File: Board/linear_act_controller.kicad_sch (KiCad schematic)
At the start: 16 parts, among them J3 PROG, U1 STM32F030K6Tx

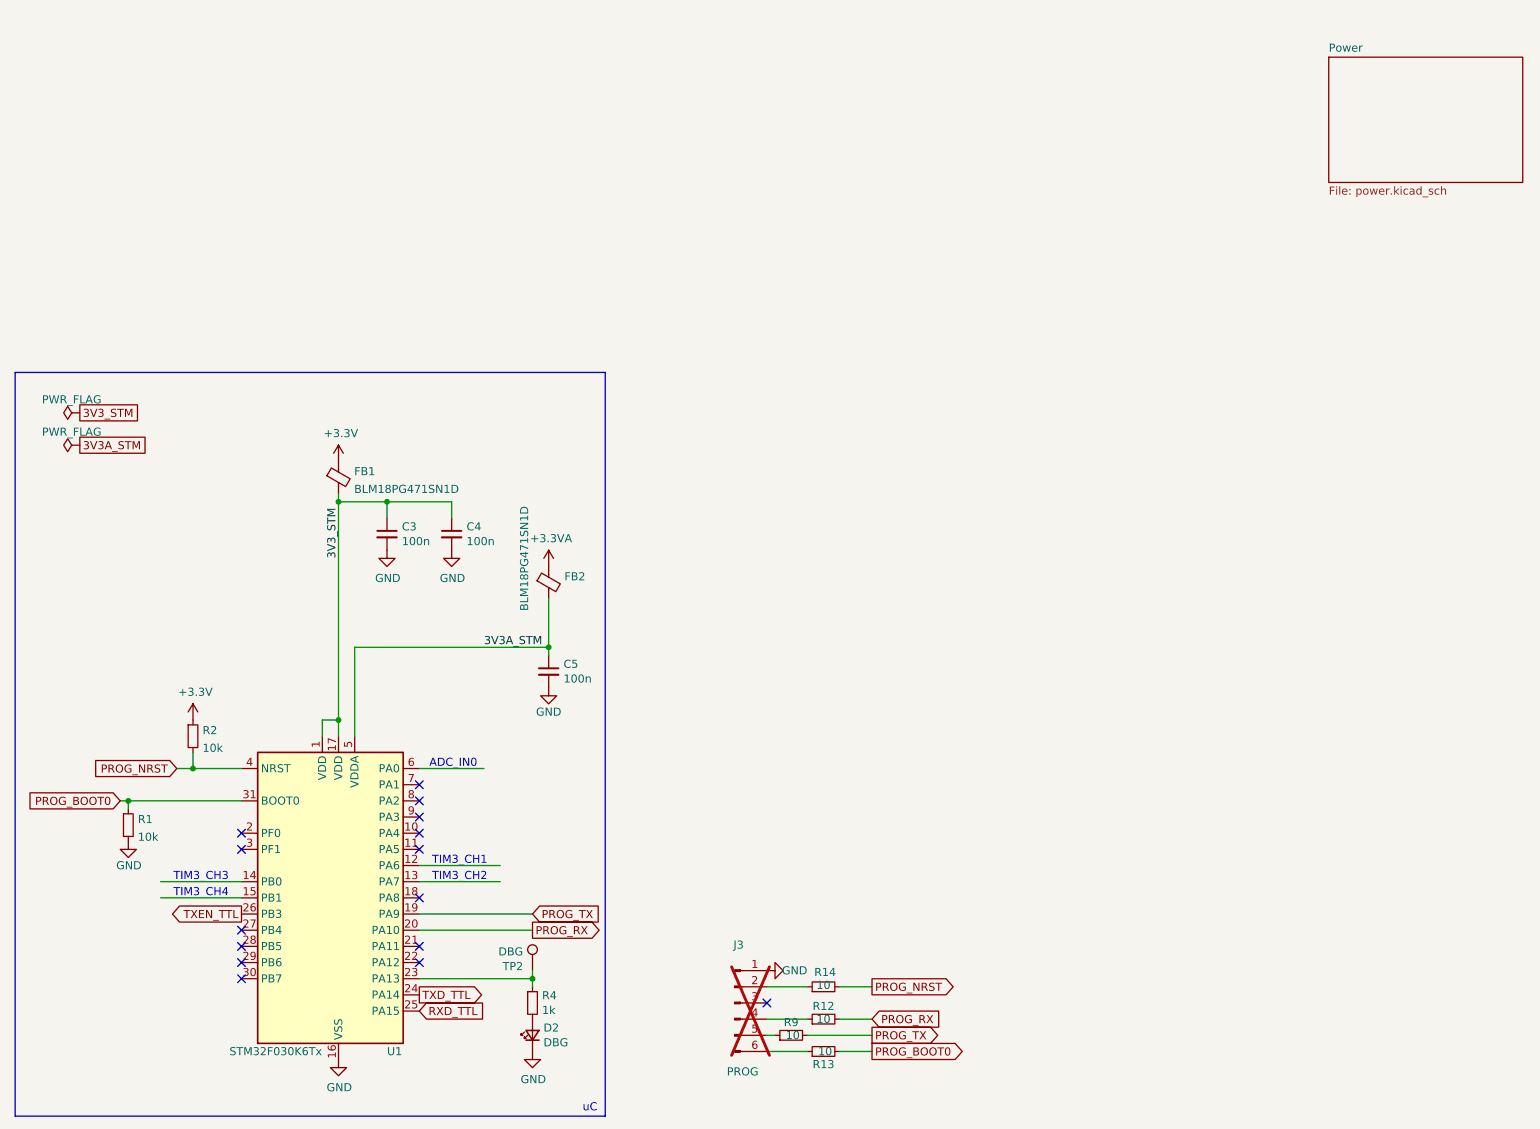
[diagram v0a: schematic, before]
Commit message: Routing mostly done
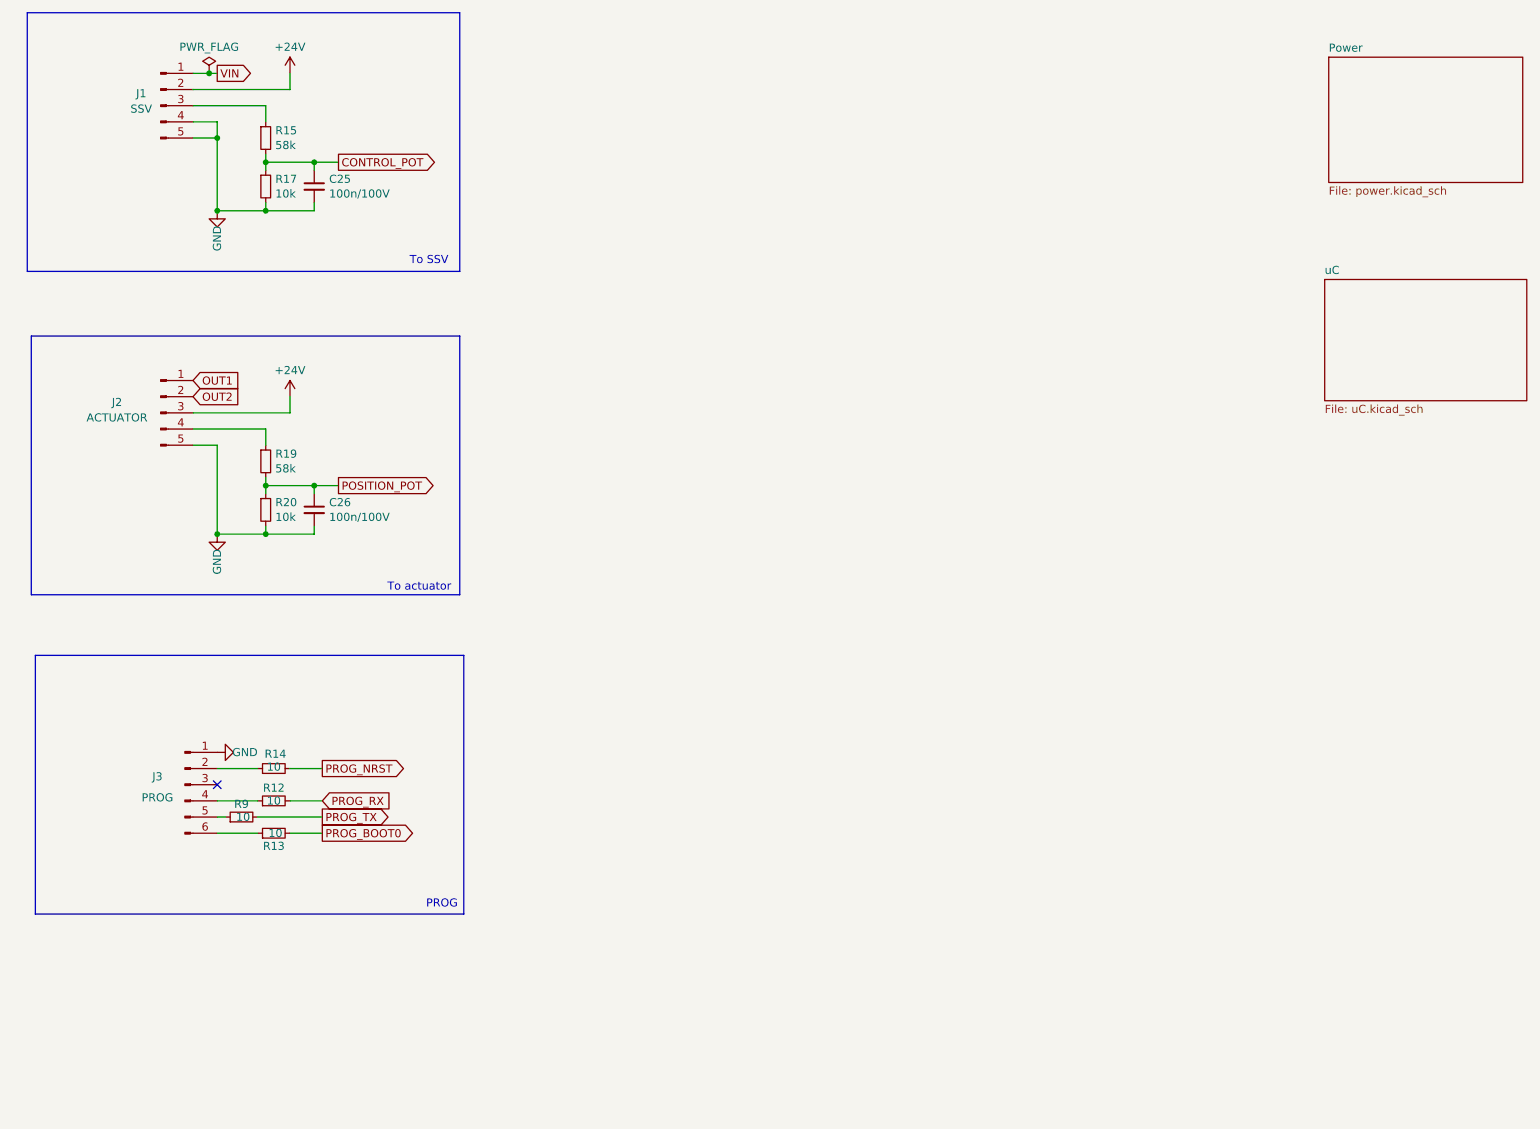
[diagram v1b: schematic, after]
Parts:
- removed C3, C4, C5: 100n, Capacitor_SMD:C_0603_1608Metric, symbol Device:C_Small
- removed D2: DBG, LED_SMD:LED_0603_1608Metric, symbol Device:LED_Small
- removed FB1, FB2: BLM18PG471SN1D, Inductor_SMD:L_0603_1608Metric, symbol Device:FerriteBead_Small
- removed R1, R2: 10k, Resistor_SMD:R_0603_1608Metric, symbol Device:R_Small
- removed R4: 1k, Resistor_SMD:R_0603_1608Metric, symbol Device:R_Small
- removed TP2: DBG, TestPoint:TestPoint_Pad_D1.0mm, symbol Connector:TestPoint
- removed U1: STM32F030K6Tx, Package_QFP:LQFP-32_7x7mm_P0.8mm, symbol MCU_ST_STM32F0:STM32F030K6Tx
- added C25, C26: 100n/100V, Capacitor_SMD:C_0603_1608Metric, symbol Device:C_Small
- added J1: SSV, symbol Connector:Conn_01x05_Pin
- added J2: ACTUATOR, symbol Connector:Conn_01x05_Pin
- added R15, R19: 58k, Resistor_SMD:R_0603_1608Metric, symbol Device:R_Small
- added R17, R20: 10k, Resistor_SMD:R_0603_1608Metric, symbol Device:R_Small
- J3: now fitted
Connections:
- net GND: now also C25.2, C26.2, J1.4 (Pin_4), J1.5 (Pin_5), J2.5 (Pin_5), R17.2, R20.2
- new net: J2.4 (Pin_4), R19.1
- new net: J1.3 (Pin_3), R15.1
- new net +24V: J1.2 (Pin_2), J2.3 (Pin_3)
- new net CONTROL_POT: C25.1, R15.2, R17.1
- new net OUT1: J2.1 (Pin_1)
- new net OUT2: J2.2 (Pin_2)
- new net POSITION_POT: C26.1, R19.2, R20.1
- new net VIN: J1.1 (Pin_1)
- no-connect marks 15 -> 1
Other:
- added sheet uC (uC.kicad_sch)
- note added: "PROG"
- note added: "To SSV"
- note added: "To actuator"
- note removed: "ADC_IN0"
- note removed: "TIM3_CH1"
- note removed: "TIM3_CH2"
- note removed: "TIM3_CH3"
- note removed: "TIM3_CH4"
- note removed: "uC"
- moved on the sheet: R12, R13, R14, R9
